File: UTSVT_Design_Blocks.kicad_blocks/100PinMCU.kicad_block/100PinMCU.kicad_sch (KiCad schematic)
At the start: 25 parts, among them SW1 SW_SPDT, U1 STM32G491VET6, U8 74AHC1G32, Y1 Crystal

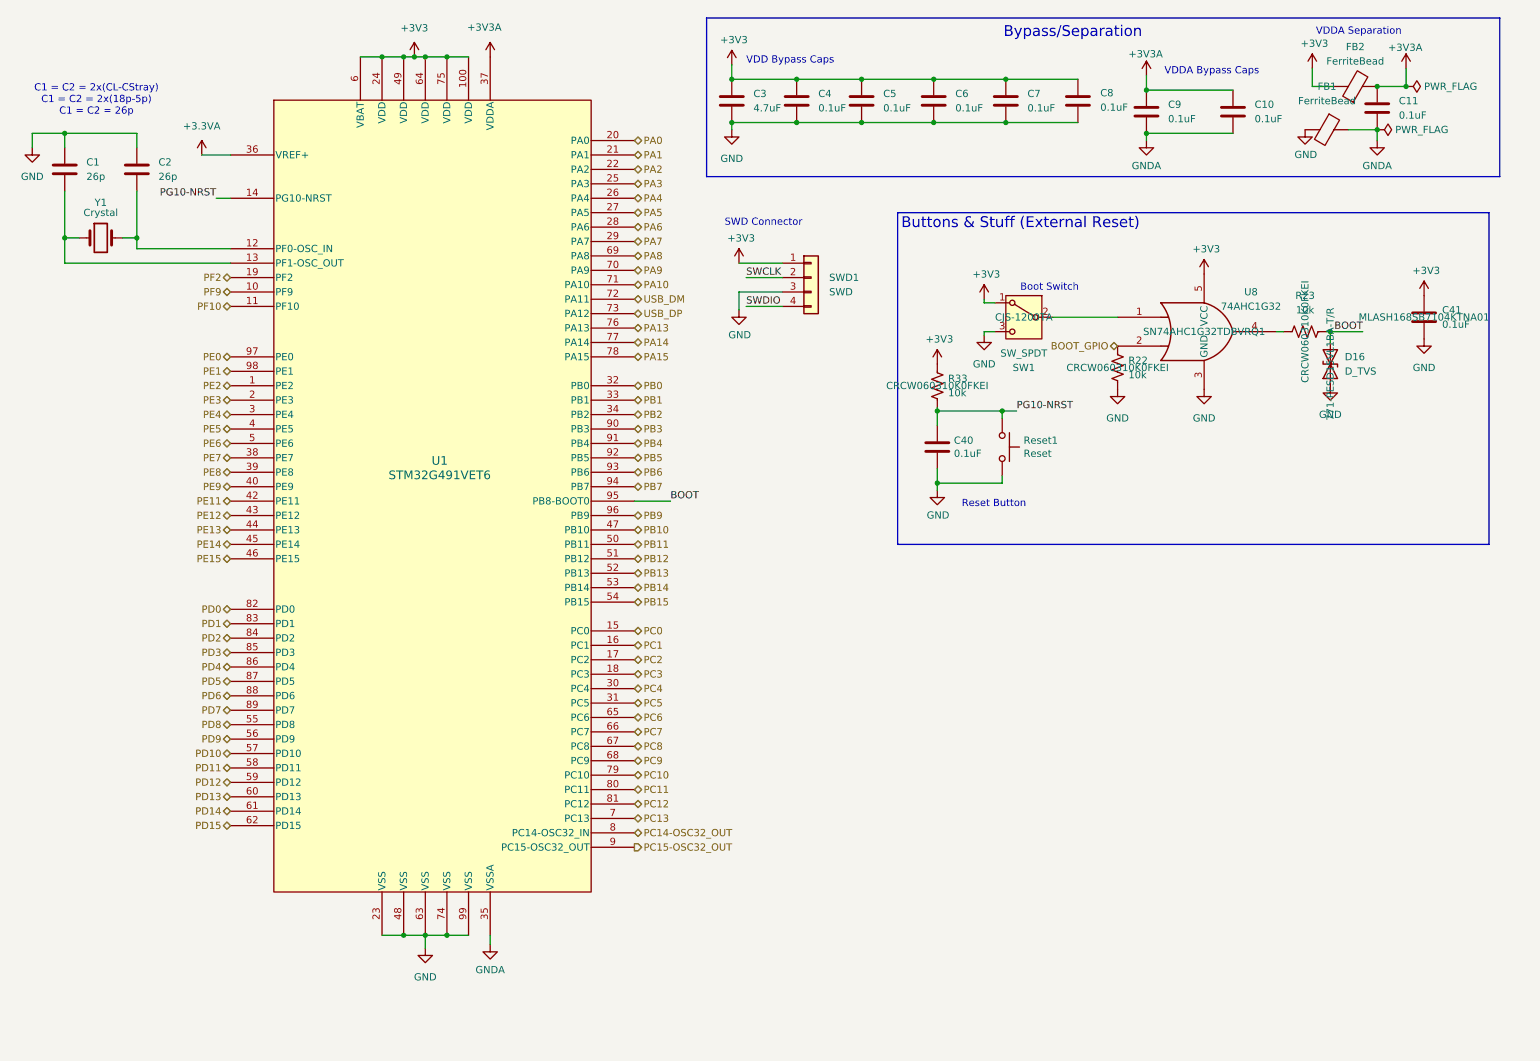
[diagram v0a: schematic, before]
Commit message: dog food
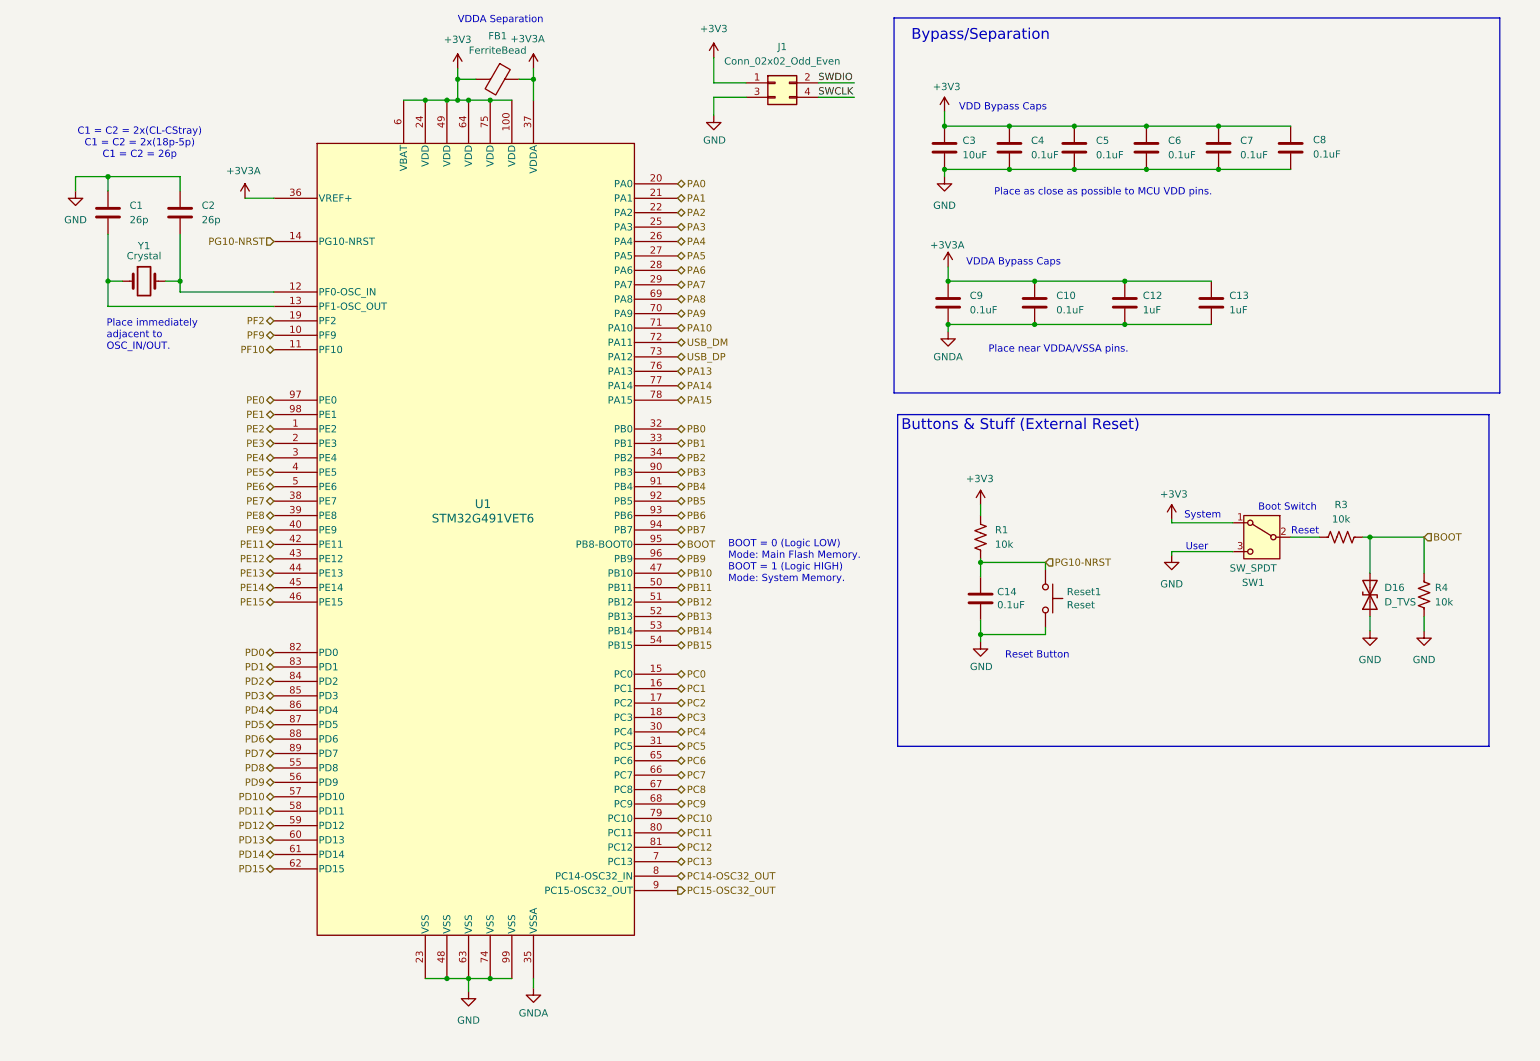
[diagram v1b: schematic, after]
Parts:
- removed C11, C41: 0.1uF, Capacitor_SMD:C_0603_1608Metric_Pad1.08x0.95mm_HandSolder, symbol Device:C
- removed FB2: FerriteBead, Inductor_SMD:L_0603_1608Metric_Pad1.05x0.95mm_HandSolder, symbol Device:FerriteBead
- removed R22: 10k, Resistor_SMD:R_0603_1608Metric_Pad0.98x0.95mm_HandSolder, symbol Device:R_US
- removed SWD1: SWD, UTSVT_Connectors:Molex_Nano-Fit_105309-xx04_1x04_P2.50mm_Vertical, symbol Connector_Generic:Conn_01x04
- removed U8: 74AHC1G32, Package_TO_SOT_SMD:SOT-23-5, symbol 74xGxx:74AHC1G32
- added C12, C13: 1uF, Capacitor_SMD:C_0603_1608Metric_Pad1.08x0.95mm_HandSolder, symbol Device:C
- added J1: Conn_02x02_Odd_Even, 878320406:CONN04_878320406_MOL, symbol Connector_Generic:Conn_02x02_Odd_Even
- added R4: 10k, Resistor_SMD:R_0603_1608Metric_Pad0.98x0.95mm_HandSolder, symbol Device:R_US
- C1, C2: footprint (none) -> Capacitor_SMD:C_0603_1608Metric_Pad1.08x0.95mm_HandSolder; P/N (none) -> 0603N270F500CT
- C3: value 4.7uF -> 10uF
- SW1: footprint UTSVT_Special:SW_CJS-1200TA -> JS102011SCQN:SWITCH_1SCQN; Mouser Part Number CJS-1200TA -> (none); P/N (none) -> JS202011JCQN
- Y1: P/N (none) -> ABM3-8.000MHZ-D2Y-T
- renumbered C40 to C14, R33 to R1, R23 to R3
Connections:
- net +3.3VA is gone; now on net +3V3A: U1.36 (VREF+)
- net +3V3: now also FB1.2, J1.1 (Pin_1)
- net +3V3A: now also FB1.1, C12.1, C13.1
- net BOOT: now also R4.2
- net GND: now also J1.3 (Pin_3), R4.1; no longer FB1.2
- net GNDA: now also C12.2, C13.2; no longer FB1.1
- net SWCLK: now also J1.4 (Pin_4)
- net SWDIO: now also J1.2 (Pin_2)
- net at SW1.2 (B): now also R3.1
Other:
- note added: "BOOT = 0 (Logic LOW) Mode: Main Flash Memory. BOOT = 1 (Logic HIGH) Mode: System Memory."
- note added: "Place as close as possible to MCU VDD pins."
- note added: "Place immediately adjacent to OSC_IN/OUT."
- note added: "Place near VDDA/VSSA pins."
- note added: "Reset"
- note added: "System"
- note added: "User"
- note removed: "SWD Connector"
- moved on the sheet: C1, C10, C14, C2, C3, C4, C5, C6, C7, C8, C9, D16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

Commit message: lakshay comments addressed
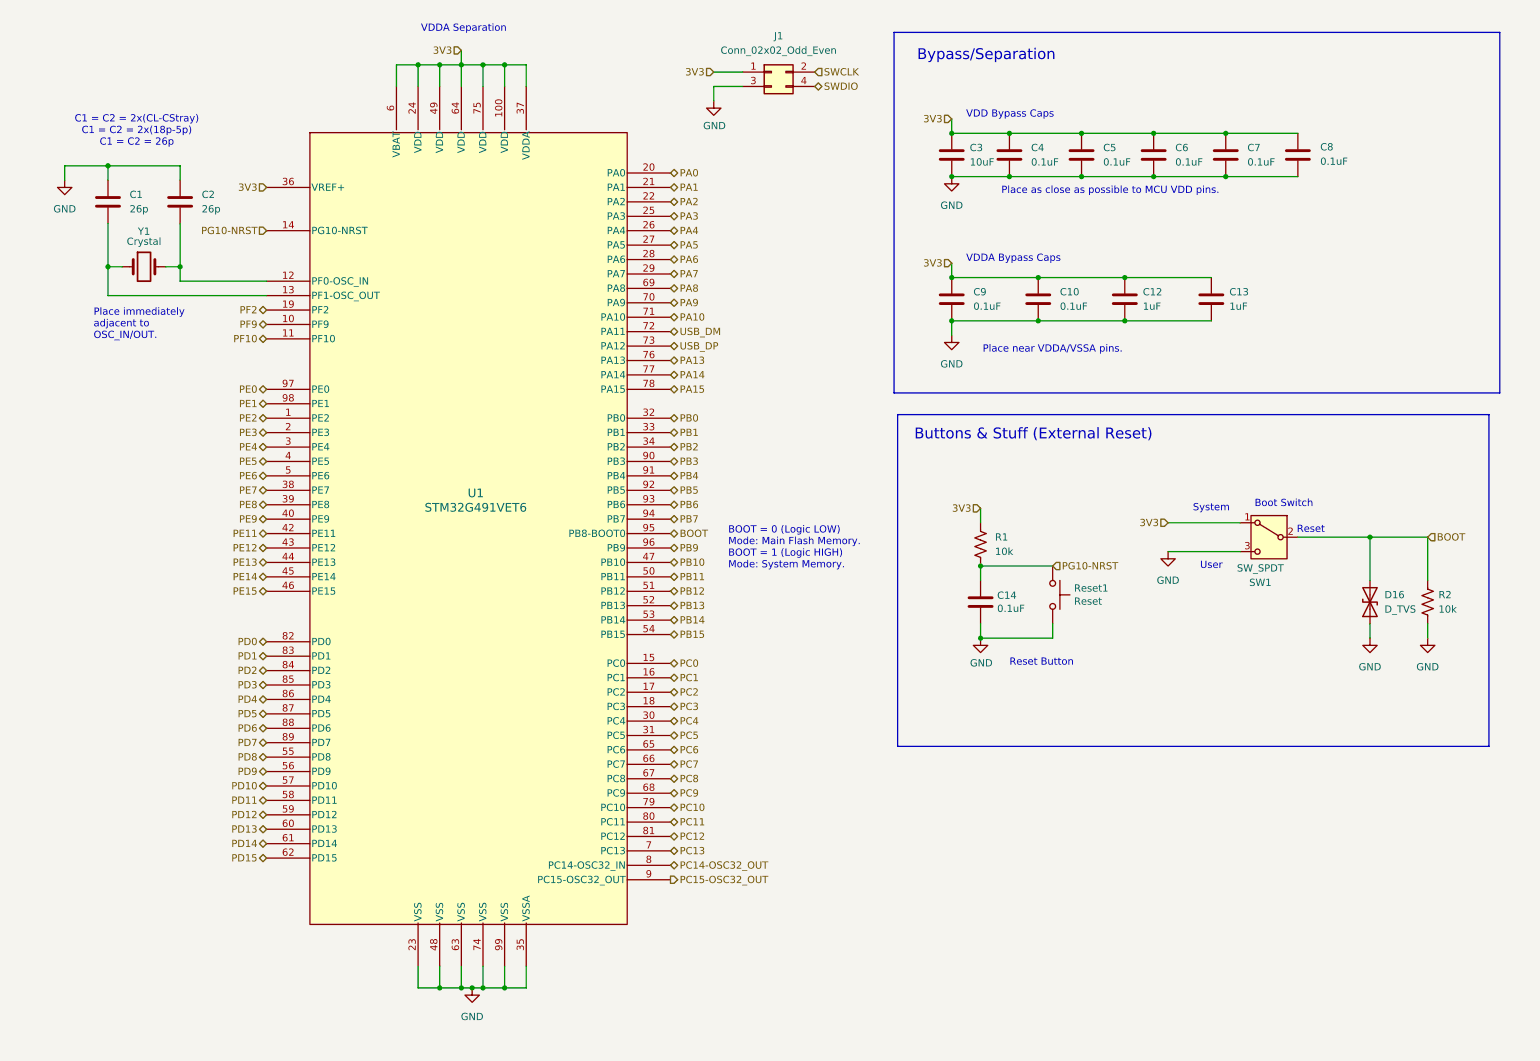
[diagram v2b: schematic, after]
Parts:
- removed FB1: FerriteBead, Inductor_SMD:L_0603_1608Metric_Pad1.05x0.95mm_HandSolder, symbol Device:FerriteBead
- removed R3: 10k, Resistor_SMD:R_0603_1608Metric_Pad0.98x0.95mm_HandSolder, symbol Device:R_US
- U1: LSCS P/N (none) -> STM32G491VET6; Mouser Part Number (none) -> 511-STM32G491VET6
- renumbered R4 to R2
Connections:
- net +3V3A is gone; now on net 3V3: C10.1, C12.1, C13.1, C9.1, U1.36 (VREF+), U1.37 (VDDA)
- net GNDA is gone; now on net GND: C10.2, C12.2, C13.2, C9.2, U1.35 (VSSA)
- net BOOT: now also SW1.2 (B)
- net SWCLK: now also J1.2 (Pin_2); no longer J1.4 (Pin_4)
- net SWDIO: now also J1.4 (Pin_4); no longer J1.2 (Pin_2)
- net +3V3 renamed 3V3
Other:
- moved on the sheet: C1, C10, C12, C13, C14, C2, C3, C4, C5, C6, C7, C8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

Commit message: post 319 brain fried stuff
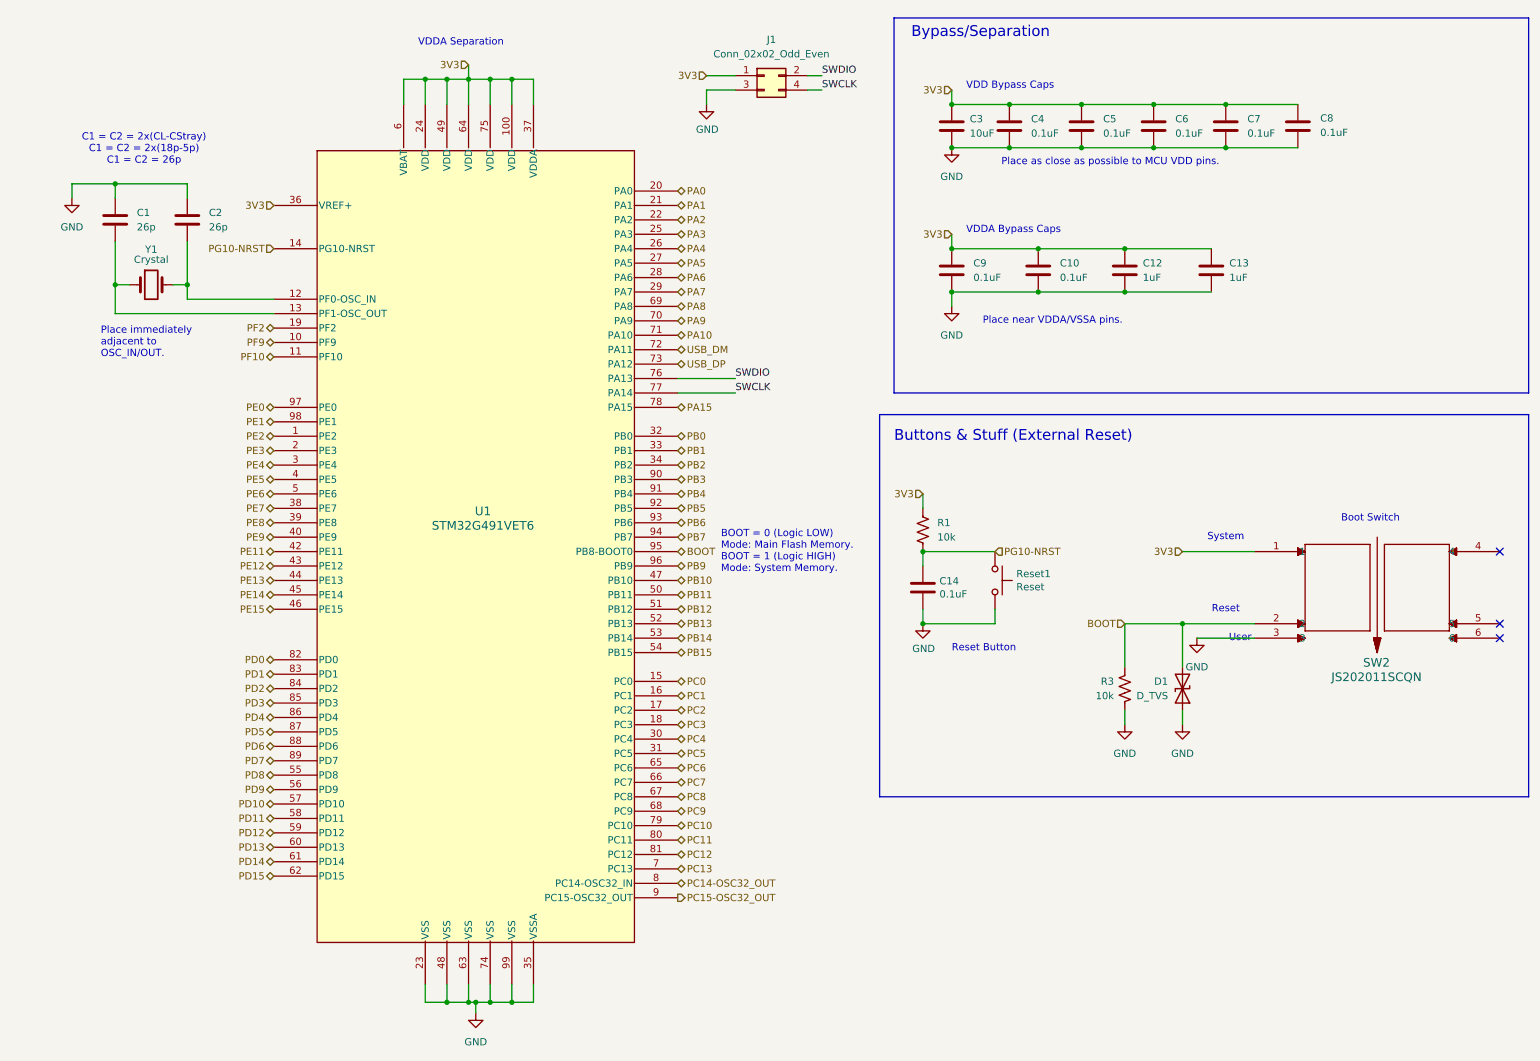
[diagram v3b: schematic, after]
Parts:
- removed D16: D_TVS, Diode_SMD:D_SOD-323, symbol Device:D_TVS
- removed R2: 10k, Resistor_SMD:R_0603_1608Metric_Pad0.98x0.95mm_HandSolder, symbol Device:R_US
- removed SW1: SW_SPDT, JS102011SCQN:SWITCH_1SCQN, symbol Switch:SW_SPDT
- added D1: D_TVS, Diode_SMD:D_SOD-323, symbol Device:D_TVS
- added R3: 10k, Resistor_SMD:R_0603_1608Metric_Pad0.98x0.95mm_HandSolder, symbol Device:R_US
- added SW2: JS202011SCQN, SW_JS202011SCQN, symbol 6pinswitch:JS202011SCQN
- C1: LCSC P/N (none) -> C92670
- C10, C14, C4, C5, C6, C7, C8, C9: LCSC P/N (none) -> C14663; P/N C0805C104M5RACTU -> MLASH168SB7104KTNA01
- C12, C13: LCSC P/N (none) -> C15849; P/N C0805C104M5RACTU -> MLASU168SB5105KTNA01
- C2: LCSC P/N (none) -> C92670; P/N 0603N270F500CT -> 0603N270F500CT
- C3: LCSC P/N (none) -> C440198; P/N GRM219R6YA475KA73D -> GRM21BR61H106KE43K
- J1: LCSC P/N (none) -> C17492485
- R1: LCSC P/N (none) -> C25804; P/N (none) -> CRCW060310K0FKEI
- Reset1: LCSC P/N (none) -> C2886926
- U1: LCSC P/N (none) -> C3209873; LSCS P/N STM32G491VET6 -> (none); Mouser Part Number 511-STM32G491VET6 -> (none); P/N (none) -> STM32G491VET6
- Y1: LCSC P/N (none) -> C144380
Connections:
- net PA13 is gone; now on net SWDIO: U1.76 (PA13)
- net PA14 is gone; now on net SWCLK: U1.77 (PA14)
- net 3V3: now also SW2.1
- net BOOT: now also D1.2 (A2), R3.2, SW2.2
- net GND: now also D1.1 (A1), R3.1, SW2.3
- net SWCLK: now also J1.4 (Pin_4); no longer J1.2 (Pin_2)
- net SWDIO: now also J1.2 (Pin_2); no longer J1.4 (Pin_4)
- no-connect marks 0 -> 3
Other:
- moved on the sheet: C1, C10, C12, C13, C14, C2, C3, C4, C5, C6, C7, C8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
